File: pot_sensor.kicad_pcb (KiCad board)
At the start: 2 copper layers, 126 x 39.5 mm, 55 parts, among them J1 USB_C_Receptacle_USB2.0_14P, SW1 EN, SW2 BOOT, U1 ESP32-C3, U2 BQ24074RGT, U3 TPS63900, U4 W25Q80DVSNIG, U5 USBLC6-2P6, U7 HDC3020DEFR, U8 TPS22917DBV, Y1 ABM8-40MHZ

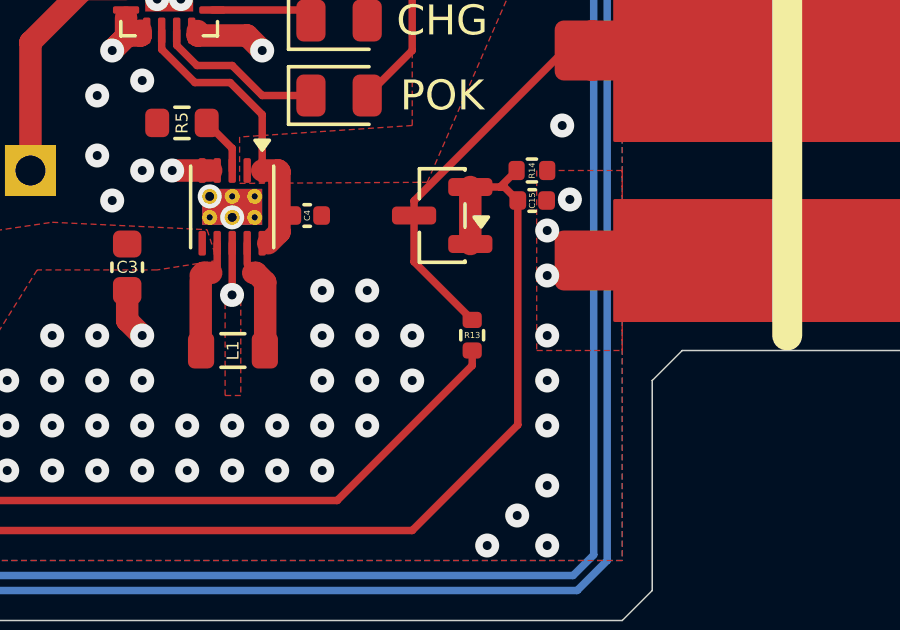
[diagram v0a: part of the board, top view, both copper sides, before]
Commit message: Finished and bought
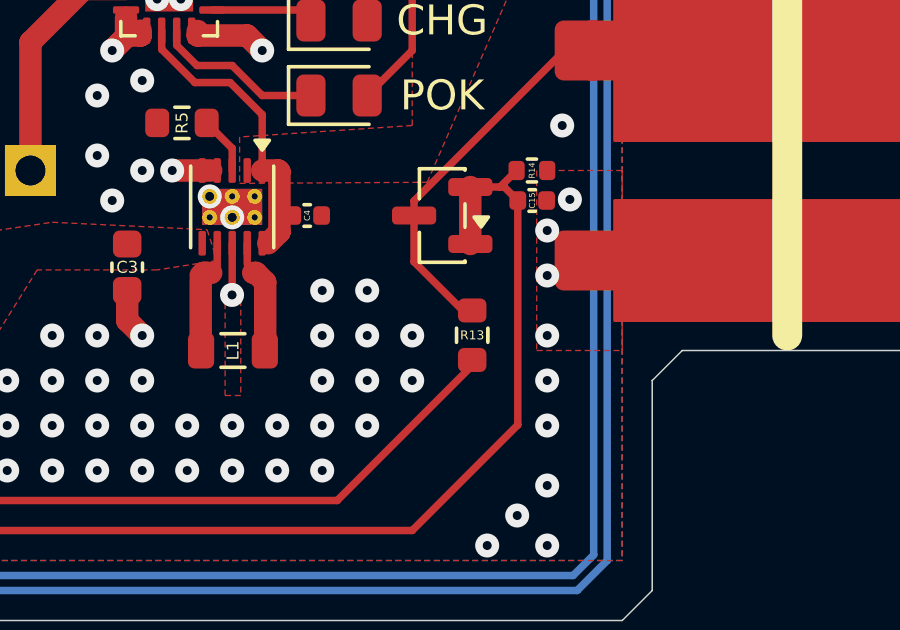
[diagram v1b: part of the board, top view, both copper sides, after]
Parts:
- D3: value BAT54A -> BAT54
- R13: footprint Resistor_SMD:R_0402_1005Metric -> Resistor_SMD:R_0603_1608Metric
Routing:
- net /1MHz_PWM: track 40.4 -> 39.9 mm
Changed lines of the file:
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@@
 			)
 		)
-		(property "Value" "BAT54A"
+		(property "Value" "BAT54"
 			(at 0 2.4 0)
 			(layer "F.Fab")
@@
 		)
 	)
-	(footprint "Resistor_SMD:R_0402_1005Metric"
+	(footprint "Resistor_SMD:R_0603_1608Metric"
 		(layer "F.Cu")
 		(at 105.5 80.49 -90)
-		(descr "Resistor SMD 0402 (1005 Metric), square (rectangular) end terminal, IPC-7351 nominal, (Body size source: IPC-SM-782 page 72, https://www.pcb-3d.com/wordpress/wp-content/uploads/ipc-sm-782a_amendment_1_and_2.pdf)")
+		(descr "Resistor SMD 0603 (1608 Metric), square (rectangular) end terminal, IPC-7351 nominal, (Body size source: IPC-SM-782 page 72, https://www.pcb-3d.com/wordpress/wp-content/uploads/ipc-sm-782a_amendment_1_and_2.pdf)")
 		(tags "resistor")
 		(property "Reference" "R13"
-			(at 0 0 180)
+			(at 0 0 0)
 			(layer "F.SilkS")
 			(effects
 				(font
-					(size 0.2 0.2)
+					(size 0.3 0.3)
 					(thickness 0.15)
 				)
@@
 		)
 		(property "Value" "10k"
-			(at 0 1.17 90)
+			(at 0 1.43 270)
 			(layer "F.Fab")
 			(effects
@@
 		)
 		(property "Datasheet" ""
-			(at 0 0 90)
+			(at 0 0 270)
 			(layer "F.Fab")
 			(hide yes)
@@
 		)
 		(property "Description" "Resistor"
-			(at 0 0 90)
+			(at 0 0 270)
 			(layer "F.Fab")
 			(hide yes)
@@
 		)
 		(property "KiLib_Generator" "SMD_2terminal_chip_molded"
-			(at 0 0 90)
-			(layer "F.SilkS")
-			(hide yes)
-			(effects
-				(font
-					(size 1 1)
-					(thickness 0.15)
-				)
-			)
-		)
-		(property "PartNumber" "ESR01MZPF1002"
 			(at 0 0 270)
-			(unlocked yes)
-			(layer "F.Fab")
+			(layer "F.SilkS")
 			(hide yes)
 			(effects
@@
 			)
 		)
-		(property "LCSC Part #" "C25744"
+		(property "LCSC Part #" "C25804"
 			(at 0 0 270)
 			(unlocked yes)
@@
 		(duplicate_pad_numbers_are_jumpers no)
 		(fp_line
-			(start -0.153641 0.38)
-			(end 0.153641 0.38)
+			(start -0.237258 0.5225)
+			(end 0.237258 0.5225)
 			(stroke
 				(width 0.12)
@@
 		)
 		(fp_line
-			(start -0.153641 -0.38)
-			(end 0.153641 -0.38)
+			(start -0.237258 -0.5225)
+			(end 0.237258 -0.5225)
 			(stroke
 				(width 0.12)
@@
 		)
 		(fp_rect
-			(start -0.93 -0.47)
-			(end 0.93 0.47)
+			(start -1.48 -0.73)
+			(end 1.48 0.73)
 			(stroke
 				(width 0.05)
@@
 		)
 		(fp_rect
-			(start -0.525 -0.27)
-			(end 0.525 0.27)
+			(start -0.8 -0.4125)
+			(end 0.8 0.4125)
 			(stroke
 				(width 0.1)
@@
 		)
 		(fp_text user "${REFERENCE}"
-			(at 0 0 90)
+			(at 0 0 270)
 			(layer "F.Fab")
 			(effects
 				(font
-					(size 0.26 0.26)
-					(thickness 0.04)
+					(size 0.4 0.4)
+					(thickness 0.06)
 				)
 			)
 		)
 		(pad "1" smd roundrect
-			(at -0.51 0 270)
-			(size 0.54 0.64)
+			(at -0.825 0 270)
+			(size 0.8 0.95)
 			(layers "F.Cu" "F.Mask" "F.Paste")
 			(roundrect_rratio 0.25)
@@
 		)
 		(pad "2" smd roundrect
-			(at 0.51 0 270)
-			(size 0.54 0.64)
+			(at 0.825 0 270)
+			(size 0.8 0.95)
 			(layers "F.Cu" "F.Mask" "F.Paste")
 			(roundrect_rratio 0.25)
@@
 		)
 		(embedded_fonts no)
-		(model "${KICAD10_3DMODEL_DIR}/Resistor_SMD.3dshapes/R_0402_1005Metric.step"
+		(model "${KICAD10_3DMODEL_DIR}/Resistor_SMD.3dshapes/R_0603_1608Metric.step"
 			(offset
 				(xyz 0 0 0)
@@
 	)
 	(segment
-		(start 105.5 79.98)
+		(start 105.185 79.665)
 		(end 103.5625 78.0425)
 		(width 0.25)
@@
 	)
 	(segment
+		(start 105.5 79.665)
+		(end 105.185 79.665)
+		(width 0.25)
+		(layer "F.Cu")
+		(net "Net-(C12-CIN)")
+	)
+	(segment
 		(start 103.5625 76.011592)
 		(end 108.574092 71)
@@
 	)
 	(segment
-		(start 105.5 81.5)
-		(end 105.5 81)
-		(width 0.25)
-		(layer "F.Cu")
-		(net "/1MHz_PWM")
-	)
-	(segment
